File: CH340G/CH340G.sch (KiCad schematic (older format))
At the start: 22 parts, among them J2 Conn_01x06, P1 USB_C_Plug_USB2.0, U1 CH340G, U2 AP2127K-3.3, Y1 Crystal_GND24

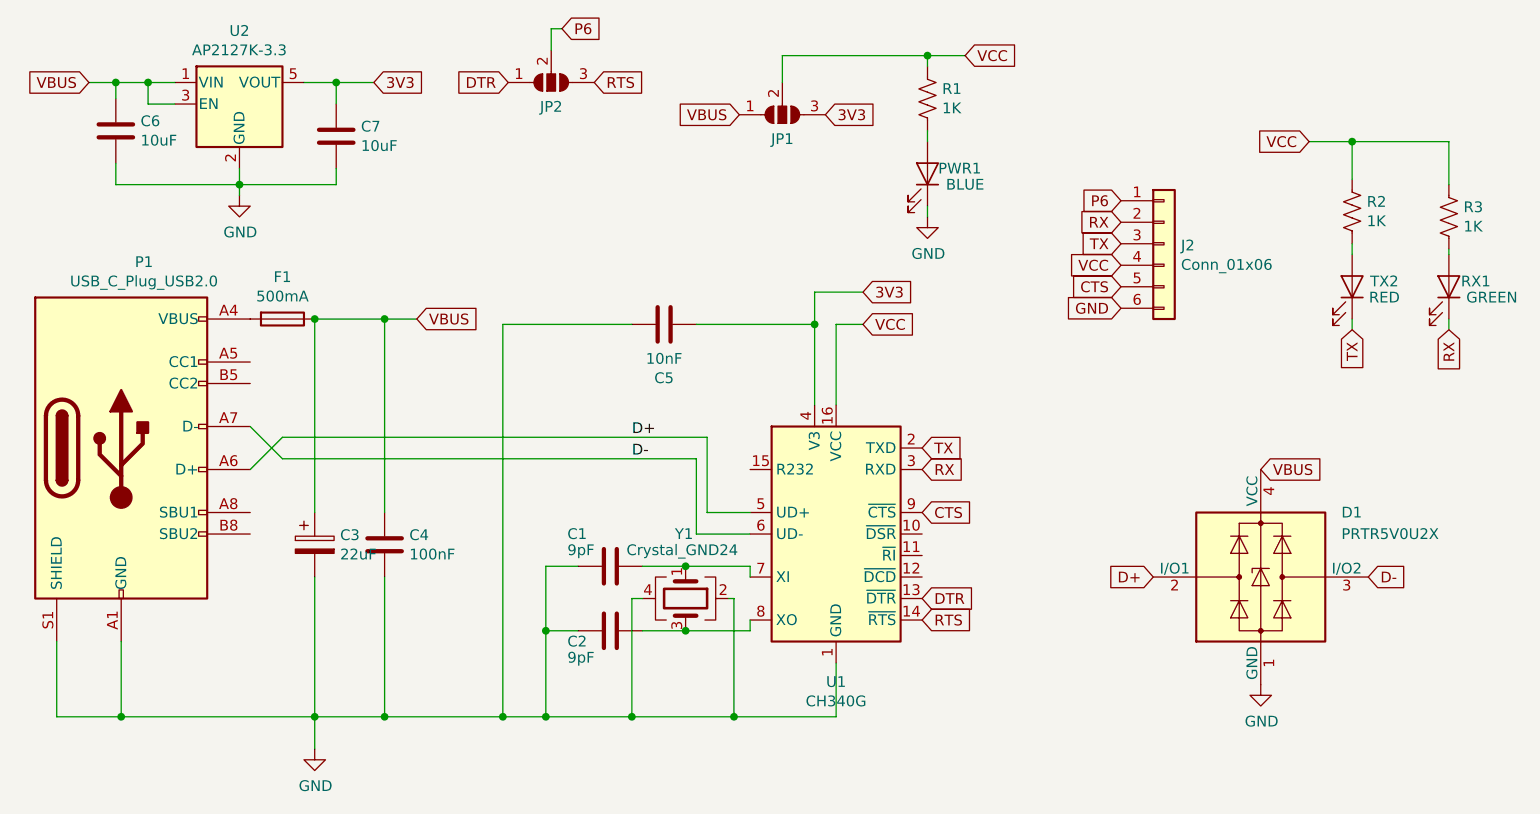
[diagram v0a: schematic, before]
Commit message: ...
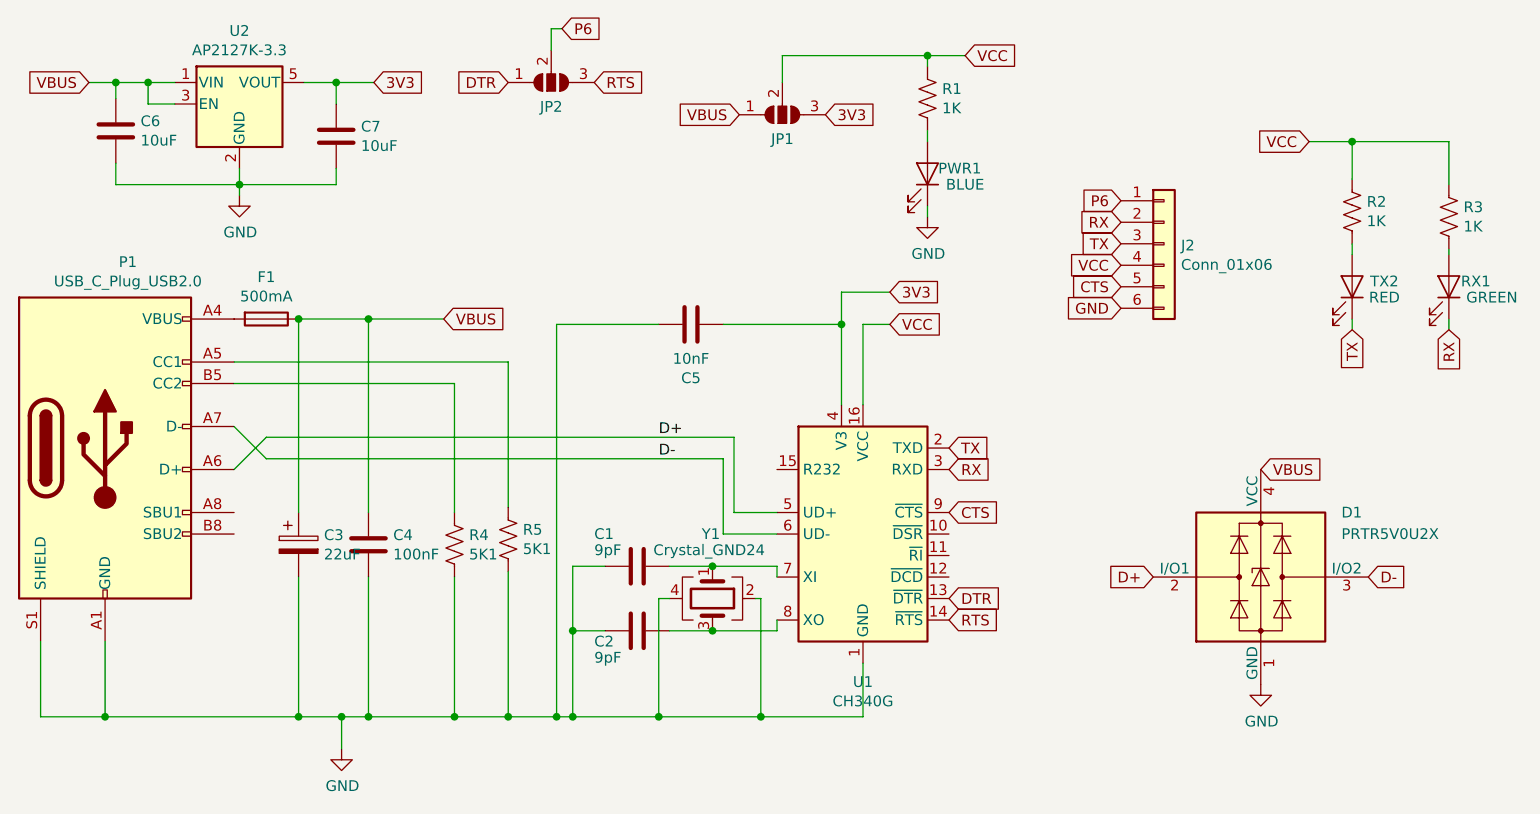
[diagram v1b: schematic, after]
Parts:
- added R4, R5: 5K1, Resistor_SMD:R_0603_1608Metric, symbol Device:R_US
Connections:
- net GND: now also R4.2, R5.2
- net at P1.A5 (CC1): now also R5.1
- net at P1.B5 (CC2): now also R4.1
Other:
- moved on the sheet: C1, C2, C3, C4, C5, F1, P1, U1, Y1
